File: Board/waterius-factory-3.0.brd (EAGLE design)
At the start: 13.5 x 60 mm, 24 parts, among them IC1 TINY13-20SU, U3 ESP01

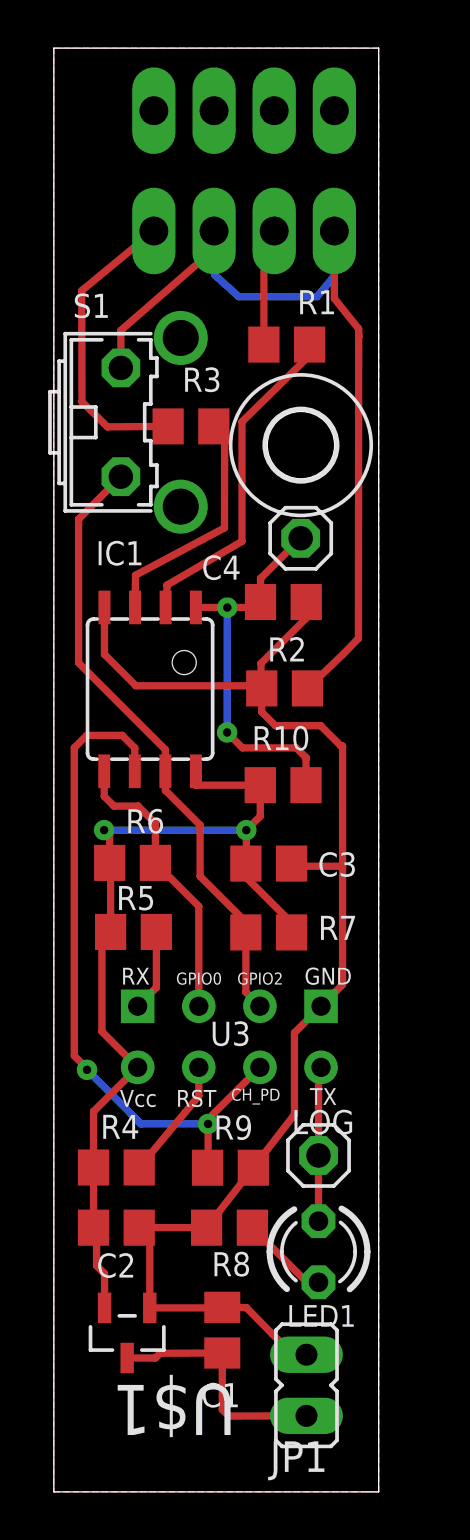
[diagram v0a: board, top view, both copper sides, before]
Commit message: board v.0.3
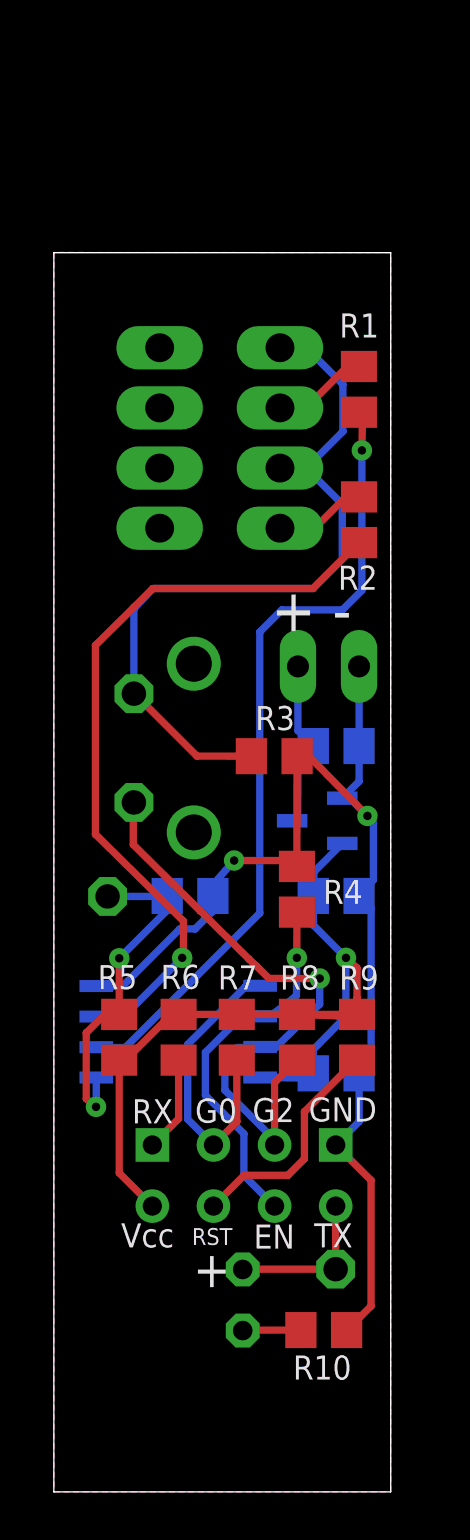
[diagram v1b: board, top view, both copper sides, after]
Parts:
- removed PAD1: MOUNT-HOLE2.8, holes:2,8
- C2: value 1uF -> 0.1uF
- C4: value 0.1uF -> 1uF
- IC1: value TINY13-20SU -> TINY85-20SU
- JP1: value + - -> (none)
- R10, R3: value 3k3 -> 300
- R2, R8: value 300 -> 3k3
- U$1: device Microchip_By_element14_Batch_1:SOT95P237X112-3N -> MCP1700T-3002E_TT:SOT95P237X112-3N
- moved JP1 29.9 mm to (11.4, 34.3), flipped to the bottom, turned to 270 degrees
- moved C1 24.7 mm to (11.7, 31.0), flipped to the bottom, turned to 180 degrees
- moved R10 22.7 mm to (11.2, 6.72)
- moved U$1 22.7 mm to (10.9, 27.9), flipped to the bottom, turned to 270 degrees
- moved C4 19.7 mm to (11.7, 17.4), flipped to the bottom, turned to 180 degrees
- moved RST 16.9 mm to (2.23, 24.7), flipped to the bottom
- moved C2 16.5 mm to (11.7, 24.8), flipped to the bottom, turned to 180 degrees
- moved IC1 14.3 mm to (5.17, 19.1), flipped to the bottom, turned to 90 degrees
- moved R3 14.1 mm to (9.16, 30.6)
- moved R4 13.8 mm to (10.1, 25.0), turned to 270 degrees
- moved S1 13.5 mm to (4.57, 30.9), flipped to the bottom, turned to 90 degrees
- moved X1 11.1 mm to (6.90, 43.8), turned to 90 degrees
- moved R8 8.39 mm to (10.1, 18.9), turned to 90 degrees
- moved R2 7.66 mm to (12.7, 40.4), turned to 270 degrees
- moved R9 7.56 mm to (12.6, 18.9), turned to 90 degrees
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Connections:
- net +3V: now also C4.1, R8.2, R9.2; no longer C3.1, R10.2, R4.2
- net GND: now also R10.1, R3.2, R4.1; no longer R2.2, R8.1, R9.1
- net GND1: now also R3.1, S1.2; no longer R2.1, S1.1
- net IN2: now also R2.2; no longer R3.2
- net N$2: now also R6.1; no longer R5.1
- net N$3: now also R9.1; no longer R4.1
- net N$4: now also C3.1, R5.1; no longer C4.1, R10.1
- net N$6: now also R10.2; no longer R8.2
- net N$8: now also R2.1; no longer R3.1
- net SCK: now also R8.1, S1.1; no longer R7.1, S1.2
- net SDA: now also R7.1; no longer R6.1
- net WAKE_UP: now also R4.2; no longer R9.2
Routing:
- net IN2: track 9.94 -> 31.9 mm, vias 0 -> 1
- net IN1: track 13.9 -> 33.4 mm, vias 0 -> 1
- net WAKE_UP: track 29.1 -> 15.7 mm, vias 2 -> 1
- net N$8: track 12.5 -> 3.83 mm
- net GND: track 57.1 -> 51.3 mm, vias 0 -> 2
- net GND1: track 37.3 -> 31.9 mm
- net N$3: track 5.06 -> 9.63 mm
- net N$1: track 10.00 -> 7.10 mm
- net N$4: track 16.9 -> 14.7 mm
- net +3V: track 38.8 -> 36.9 mm, vias 2 -> 1
- net SDA: track 12.0 -> 13.2 mm
- net N$6: track 3.69 -> 2.58 mm
- net N$7: track 4.90 -> 3.99 mm
- net N$2: track 3.41 -> 3.98 mm
- net SCK: track 25.9 -> 26.1 mm, vias 0 -> 1
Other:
- board size 13.5 x 60 mm -> 14 x 51.5 mm
- board text added: "+"
- board text added: "+ -"
- board text added: "- +"
- board text added: "EN"
- board text added: "G0"
- board text added: "G2"
- board text added: "v0.3"
- board text added: "waterius.ru"
- board text removed: "CH_PD"
- board text removed: "GPIO0"
- board text removed: "GPIO2"
- board text removed: "U3"
